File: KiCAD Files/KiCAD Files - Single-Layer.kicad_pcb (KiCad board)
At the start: 2 copper layers, 140 x 120 mm, 49 parts, among them J1 Power-Input, J10 SPI-Expansion, J11 I2C-Expansion, J12 Flow, J2 Pump-Conn, J3 Chopper-Conn, J4 Heater-Conn, J5 Term-1, J6 Term-2, J7 Humidity, J8 MQ-2-Methane, J9 MQ-135-CO2, K2 Chopper-Relay, K3 Heater-Relay, Q1 IRFZ44N, Q2 BD139, Q3 BD139, U1 Arduino_Nano_ESP32, U2 LM7805, U3 LM7808, U4 LM7812

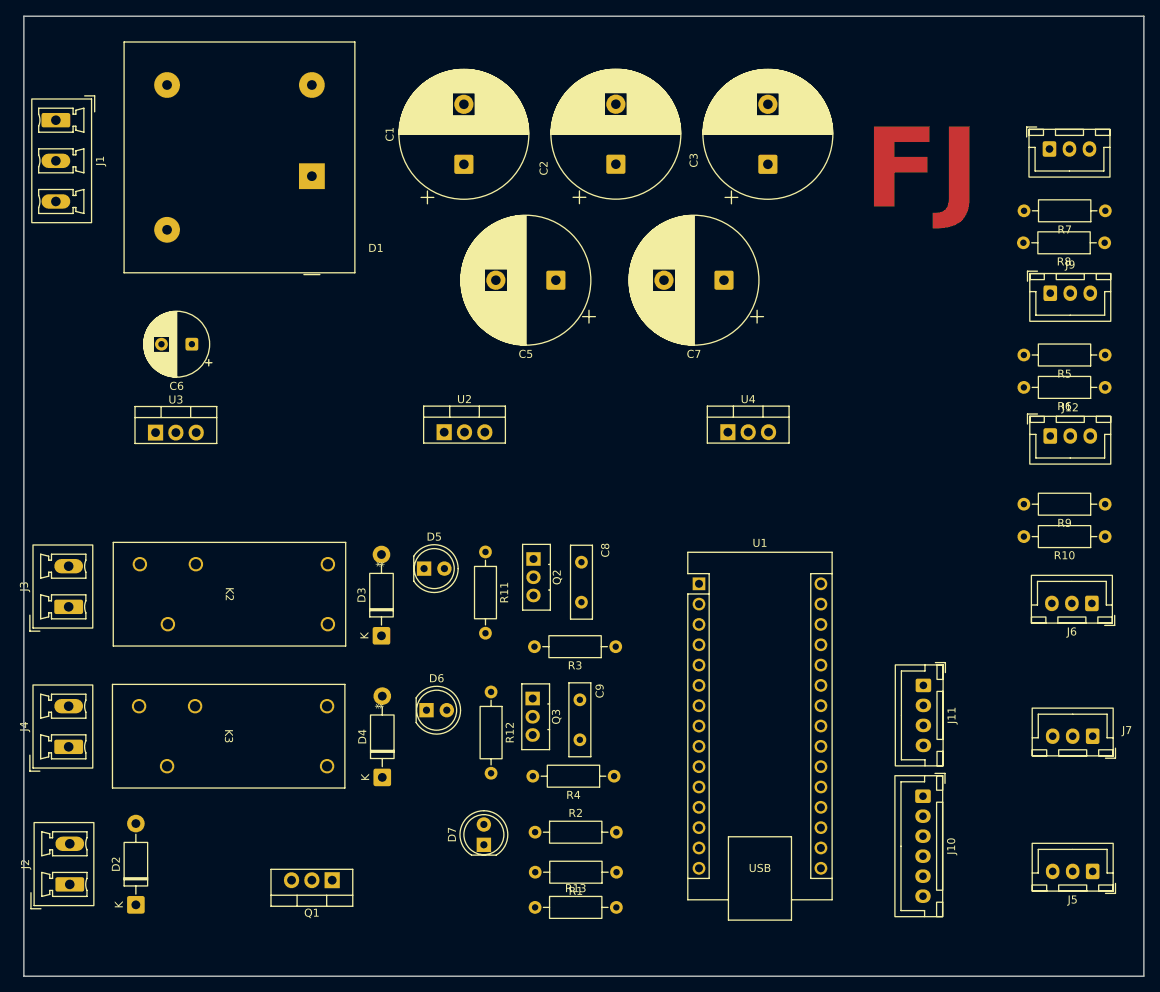
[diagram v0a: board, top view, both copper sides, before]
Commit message: Single-Layer-PCB
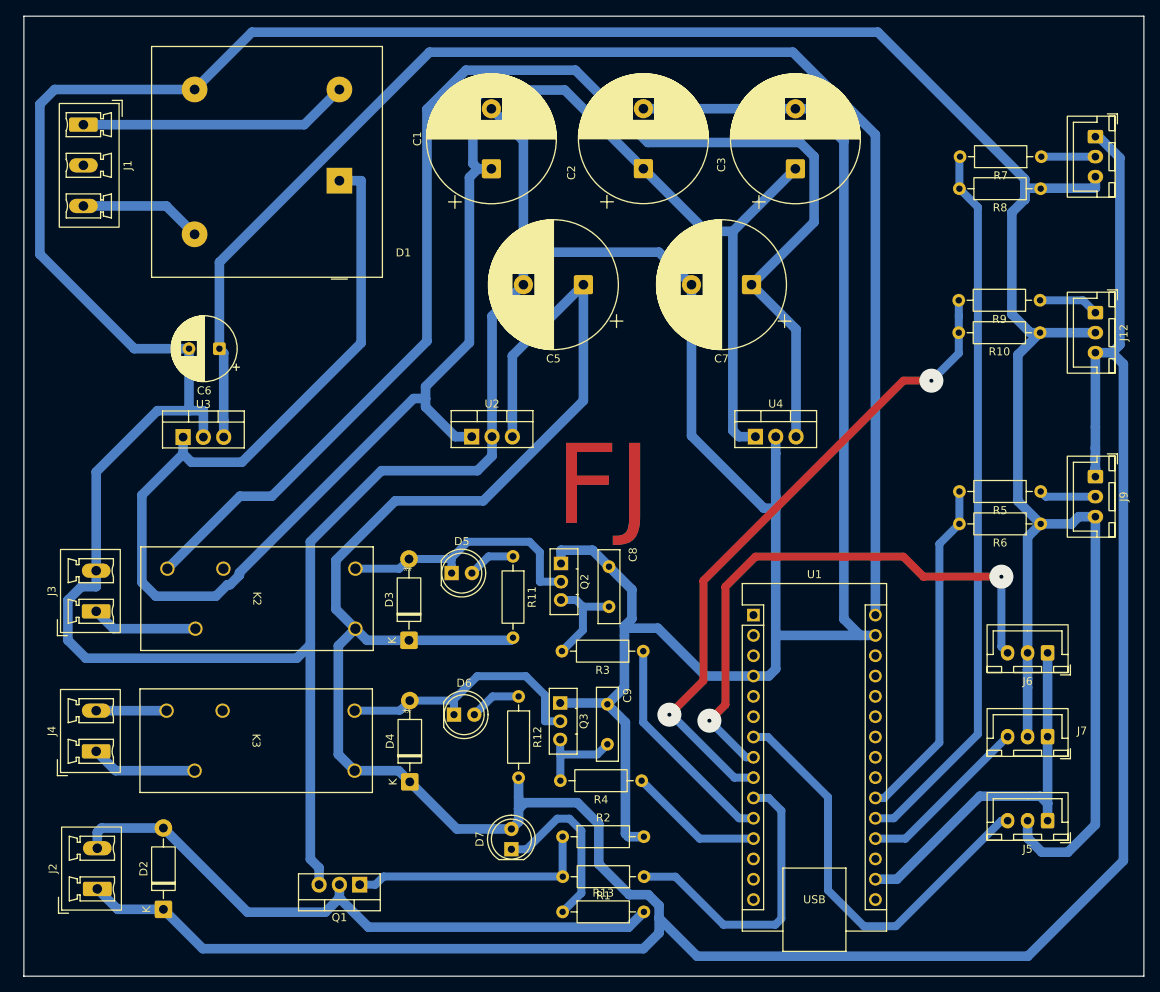
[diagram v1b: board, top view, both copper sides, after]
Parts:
- removed J10: SPI-Expansion, Connector_JST:JST_XH_B6B-XH-A_1x06_P2.50mm_Vertical
- removed J11: I2C-Expansion, Connector_JST:JST_XH_B4B-XH-A_1x04_P2.50mm_Vertical
- moved R10 26.8 mm to (172.0, 79.6)
- moved R9 26.8 mm to (172.0, 75.5)
- moved J9 23.6 mm to (178.9, 97.6), turned to -90 degrees
- moved R5 18.9 mm to (172.1, 99.4)
- moved R6 18.9 mm to (172.1, 103.5)
- moved J12 16.4 mm to (178.9, 77.1), turned to -90 degrees
- moved R7 10.5 mm to (172.2, 57.6)
- moved R8 10.5 mm to (172.1, 61.6)
- moved J5 8.48 mm to (173.0, 140.6)
- moved J6 8.30 mm to (173.0, 119.6)
- moved U1 7.85 mm to (136.2, 114.9)
- moved J8 5.94 mm to (178.9, 55.1), turned to -90 degrees
- moved J7 5.64 mm to (173.0, 130.1)
- moved C7 3.49 mm to (136.0, 73.6)
- moved C1 3.49 mm to (103.4, 59.1)
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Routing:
- net GND: track 0.00 -> 792.7 mm
- net +5V: track 0.00 -> 434.5 mm
- net VS: track 0.00 -> 248.4 mm
- net +8V: track 0.00 -> 179.3 mm
- net +12V: track 0.00 -> 168.7 mm
- net /Methane: track 0.00 -> 90.3 mm
- net /Flow: track 0.00 -> 82.6 mm, vias 0 -> 2
- net Net-(D2-A): track 0.00 -> 79.6 mm
- net /Term-2: track 0.00 -> 71.9 mm, vias 0 -> 2
- net /Term-1: track 0.00 -> 53.9 mm
- net +3.3V: track 0.00 -> 47.2 mm
- net /CO2: track 0.00 -> 43.3 mm
- net /Pump: track 0.00 -> 37.6 mm
- net Net-(J1-Pin_1): track 0.00 -> 33.8 mm
- net Net-(D4-A): track 0.00 -> 33.6 mm
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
